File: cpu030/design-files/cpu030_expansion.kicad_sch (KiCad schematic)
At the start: 20 parts, among them J801 DIN41612_03x32_ABC, U801 74ACT245, U802 74ACT245, U803 74ACT245, U804 74ACT245, U805 74ACT245, U806 74ACT245, U807 74ACT245, U808 74ACT245

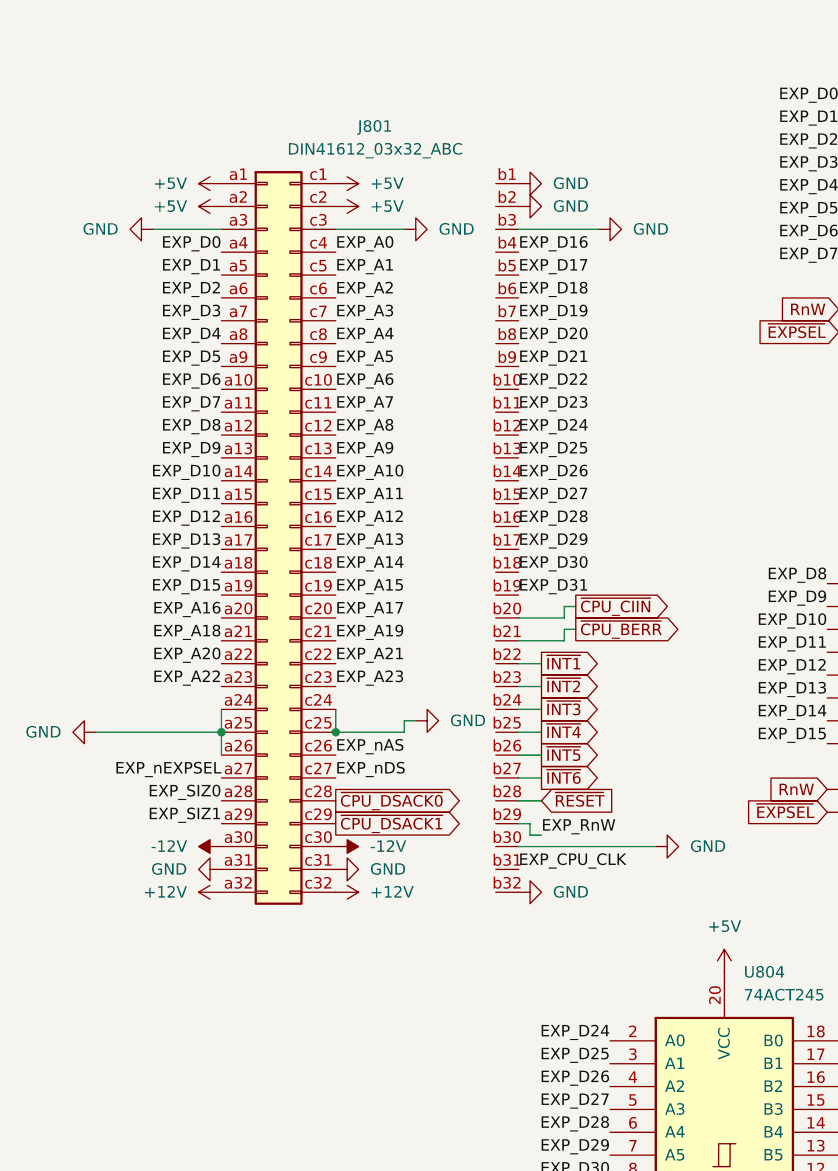
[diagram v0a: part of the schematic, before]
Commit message: Pullups on the INTx inputs.
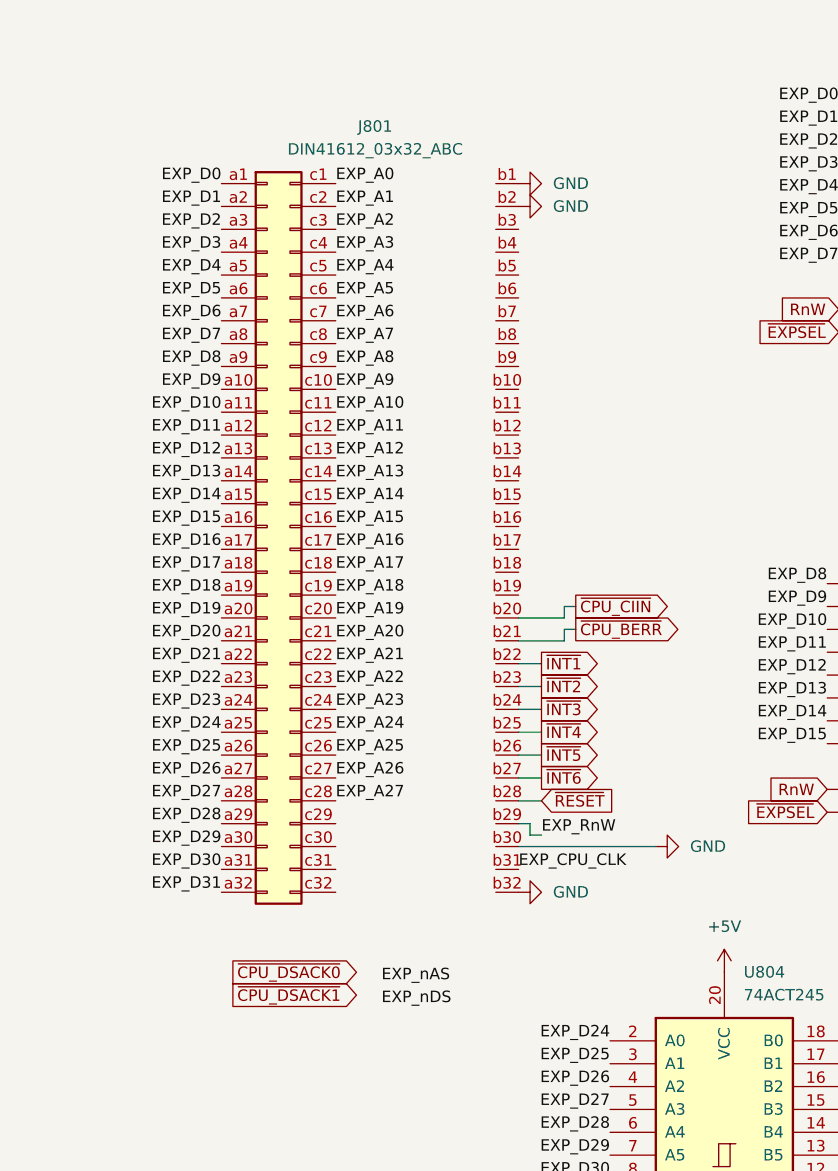
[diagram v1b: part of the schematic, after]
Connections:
- net +12V: no longer J801.a32 (Pin_a32), J801.c32 (Pin_c32)
- net +5V: no longer J801.a1 (Pin_a1), J801.a2 (Pin_a2), J801.c1 (Pin_c1), J801.c2 (Pin_c2)
- net -12V: no longer J801.a30 (Pin_a30), J801.c30 (Pin_c30)
- net EXP_A0: now also J801.c1 (Pin_c1); no longer J801.c4 (Pin_c4)
- net EXP_A1: now also J801.c2 (Pin_c2); no longer J801.c5 (Pin_c5)
- net EXP_A10: now also J801.c11 (Pin_c11); no longer J801.c14 (Pin_c14)
- net EXP_A11: now also J801.c12 (Pin_c12); no longer J801.c15 (Pin_c15)
- net EXP_A12: now also J801.c13 (Pin_c13); no longer J801.c16 (Pin_c16)
- net EXP_A13: now also J801.c14 (Pin_c14); no longer J801.c17 (Pin_c17)
- net EXP_A14: now also J801.c15 (Pin_c15); no longer J801.c18 (Pin_c18)
- net EXP_A15: now also J801.c16 (Pin_c16); no longer J801.c19 (Pin_c19)
- net EXP_A16: now also J801.c17 (Pin_c17); no longer J801.a20 (Pin_a20)
- net EXP_A17: now also J801.c18 (Pin_c18); no longer J801.c20 (Pin_c20)
- net EXP_A18: now also J801.c19 (Pin_c19); no longer J801.a21 (Pin_a21)
- net EXP_A19: now also J801.c20 (Pin_c20); no longer J801.c21 (Pin_c21)
- net EXP_A2: now also J801.c3 (Pin_c3); no longer J801.c6 (Pin_c6)
- net EXP_A20: now also J801.c21 (Pin_c21); no longer J801.a22 (Pin_a22)
- net EXP_A22: now also J801.c23 (Pin_c23); no longer J801.a23 (Pin_a23)
- net EXP_A23: now also J801.c24 (Pin_c24); no longer J801.c23 (Pin_c23)
- net EXP_A3: now also J801.c4 (Pin_c4); no longer J801.c7 (Pin_c7)
- net EXP_A4: now also J801.c5 (Pin_c5); no longer J801.c8 (Pin_c8)
- net EXP_A5: now also J801.c6 (Pin_c6); no longer J801.c9 (Pin_c9)
- net EXP_A6: now also J801.c7 (Pin_c7); no longer J801.c10 (Pin_c10)
- net EXP_A7: now also J801.c8 (Pin_c8); no longer J801.c11 (Pin_c11)
- net EXP_A8: now also J801.c9 (Pin_c9); no longer J801.c12 (Pin_c12)
- net EXP_A9: now also J801.c10 (Pin_c10); no longer J801.c13 (Pin_c13)
- net EXP_D0: now also J801.a1 (Pin_a1); no longer J801.a4 (Pin_a4)
- net EXP_D1: now also J801.a2 (Pin_a2); no longer J801.a5 (Pin_a5)
- net EXP_D10: now also J801.a11 (Pin_a11); no longer J801.a14 (Pin_a14)
- net EXP_D11: now also J801.a12 (Pin_a12); no longer J801.a15 (Pin_a15)
- net EXP_D12: now also J801.a13 (Pin_a13); no longer J801.a16 (Pin_a16)
- net EXP_D13: now also J801.a14 (Pin_a14); no longer J801.a17 (Pin_a17)
- net EXP_D14: now also J801.a15 (Pin_a15); no longer J801.a18 (Pin_a18)
- net EXP_D15: now also J801.a16 (Pin_a16); no longer J801.a19 (Pin_a19)
- net EXP_D16: now also J801.a17 (Pin_a17); no longer J801.b4 (Pin_b4)
- net EXP_D17: now also J801.a18 (Pin_a18); no longer J801.b5 (Pin_b5)
- net EXP_D18: now also J801.a19 (Pin_a19); no longer J801.b6 (Pin_b6)
- net EXP_D19: now also J801.a20 (Pin_a20); no longer J801.b7 (Pin_b7)
- net EXP_D2: now also J801.a3 (Pin_a3); no longer J801.a6 (Pin_a6)
- net EXP_D20: now also J801.a21 (Pin_a21); no longer J801.b8 (Pin_b8)
- net EXP_D21: now also J801.a22 (Pin_a22); no longer J801.b9 (Pin_b9)
- net EXP_D22: now also J801.a23 (Pin_a23); no longer J801.b10 (Pin_b10)
- net EXP_D23: now also J801.a24 (Pin_a24); no longer J801.b11 (Pin_b11)
- net EXP_D24: now also J801.a25 (Pin_a25); no longer J801.b12 (Pin_b12)
- net EXP_D25: now also J801.a26 (Pin_a26); no longer J801.b13 (Pin_b13)
- net EXP_D26: now also J801.a27 (Pin_a27); no longer J801.b14 (Pin_b14)
- net EXP_D27: now also J801.a28 (Pin_a28); no longer J801.b15 (Pin_b15)
- net EXP_D28: now also J801.a29 (Pin_a29); no longer J801.b16 (Pin_b16)
- net EXP_D29: now also J801.a30 (Pin_a30); no longer J801.b17 (Pin_b17)
- net EXP_D3: now also J801.a4 (Pin_a4); no longer J801.a7 (Pin_a7)
- net EXP_D30: now also J801.a31 (Pin_a31); no longer J801.b18 (Pin_b18)
- net EXP_D31: now also J801.a32 (Pin_a32); no longer J801.b19 (Pin_b19)
- net EXP_D4: now also J801.a5 (Pin_a5); no longer J801.a8 (Pin_a8)
- net EXP_D5: now also J801.a6 (Pin_a6); no longer J801.a9 (Pin_a9)
- net EXP_D6: now also J801.a7 (Pin_a7); no longer J801.a10 (Pin_a10)
- net EXP_D7: now also J801.a8 (Pin_a8); no longer J801.a11 (Pin_a11)
- net EXP_D8: now also J801.a9 (Pin_a9); no longer J801.a12 (Pin_a12)
- net EXP_D9: now also J801.a10 (Pin_a10); no longer J801.a13 (Pin_a13)
- net EXP_SIZ0: no longer J801.a28 (Pin_a28)
- net EXP_SIZ1: no longer J801.a29 (Pin_a29)
- net EXP_nAS: no longer J801.c26 (Pin_c26)
- net EXP_nDS: no longer J801.c27 (Pin_c27)
- net EXP_nEXPSEL: no longer J801.a27 (Pin_a27)
- net GND: no longer J801.a24 (Pin_a24), J801.a25 (Pin_a25), J801.a26 (Pin_a26), J801.a3 (Pin_a3), J801.a31 (Pin_a31), J801.b3 (Pin_b3), J801.c24 (Pin_c24), J801.c25 (Pin_c25), J801.c3 (Pin_c3), J801.c31 (Pin_c31)
- net ~{CPU_DSACK0}: no longer J801.c28 (Pin_c28)
- net ~{CPU_DSACK1}: no longer J801.c29 (Pin_c29)
- new net EXP_A24: J801.c25 (Pin_c25)
- new net EXP_A25: J801.c26 (Pin_c26)
- new net EXP_A26: J801.c27 (Pin_c27)
- new net EXP_A27: J801.c28 (Pin_c28)
